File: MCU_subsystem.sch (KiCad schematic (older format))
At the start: 14 parts, among them U601 cc1352p, U602 MX25R8035FZUIL0, Y601 32.768kHz, Y602 48MHz

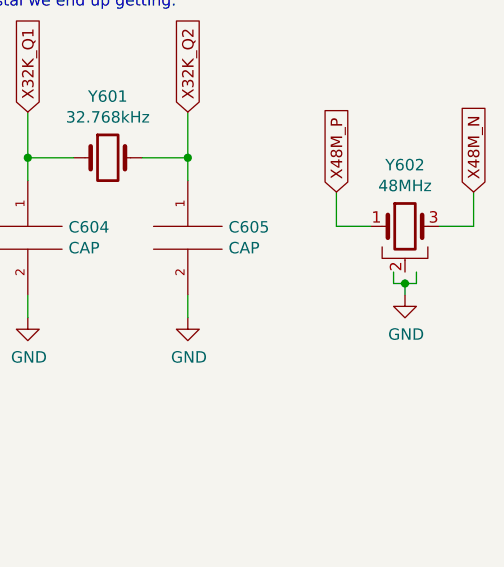
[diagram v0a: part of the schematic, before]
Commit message: Apparently the schematic wasn't saved, and thus not commited. Here's that commit.
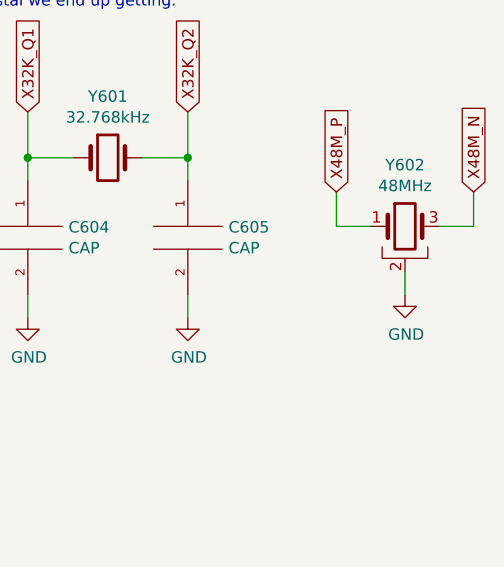
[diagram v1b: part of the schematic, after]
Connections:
- net GND: now also Y602.2
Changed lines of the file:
@@
 $EndComp
 Wire Wire Line
-	8700 4500 8700 4550
-Wire Wire Line
-	8700 4550 8750 4550
-Wire Wire Line
-	8800 4550 8800 4500
-Wire Wire Line
-	8750 4600 8750 4550
-Connection ~ 8750 4550
-Wire Wire Line
-	8750 4550 8800 4550
+	8750 4500 8750 4600
 $EndSCHEMATC
